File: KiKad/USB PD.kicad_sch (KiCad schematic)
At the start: 7 parts, among them J101 POWER_OUT, J4 USB_C_Receptacle_PowerOnly_6P, J5 USB_C_Receptacle_USB2.0_14P, Q301 Si2369, Q302 Si2338

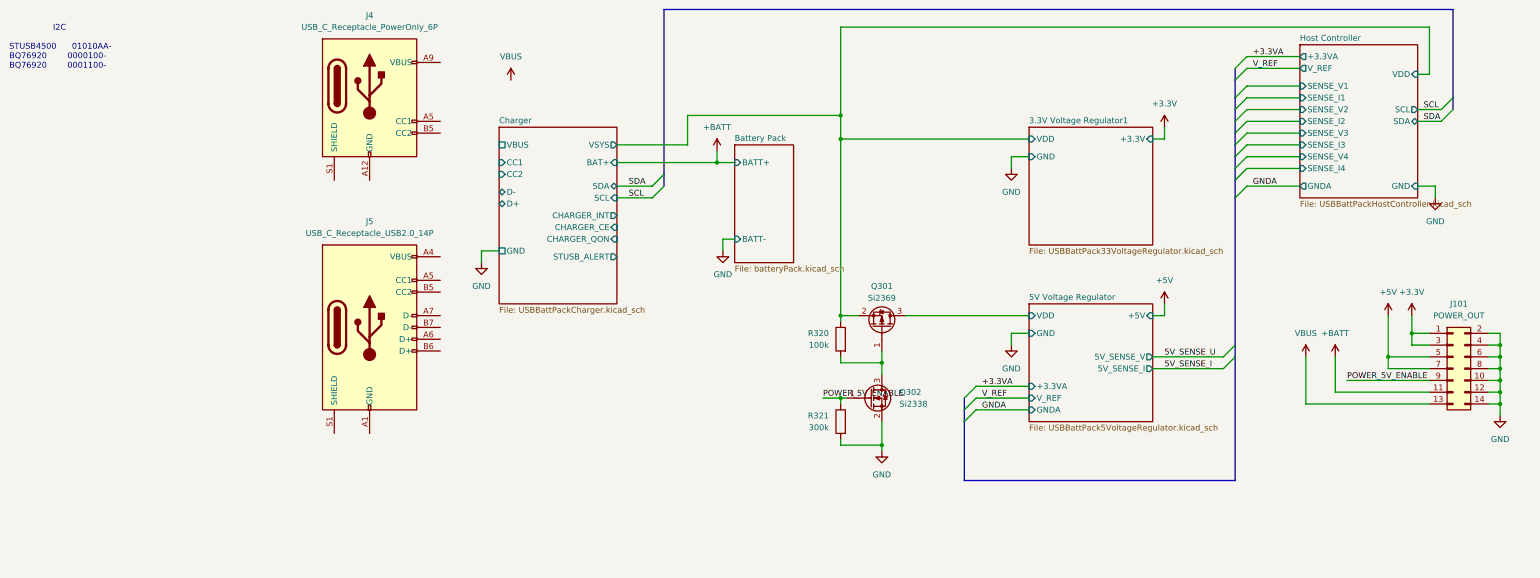
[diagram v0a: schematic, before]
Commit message: some work
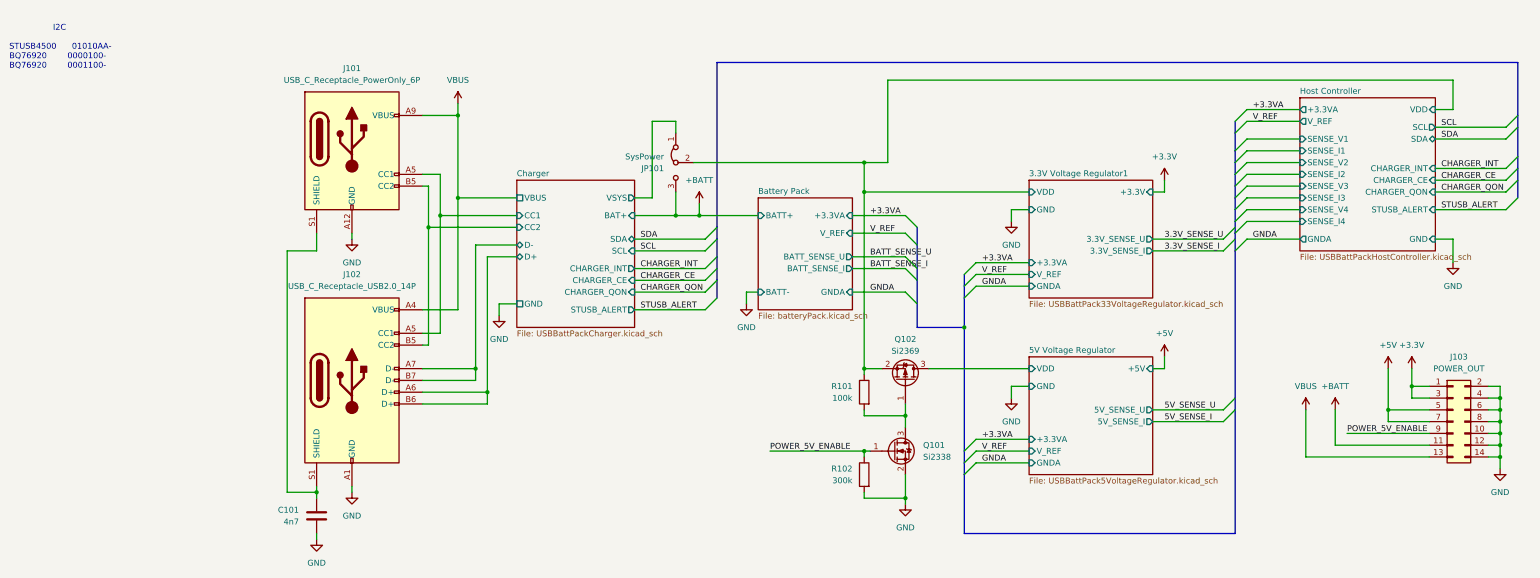
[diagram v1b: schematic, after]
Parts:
- added C101: 4n7, Capacitor_SMD:C_0805_2012Metric, symbol Device:C
- added JP101: SysPower, symbol Jumper:Jumper_3_Bridged12
- renumbered J4 to J101, J5 to J102, J101 to J103, Q302 to Q101, Q301 to Q102, R320 to R101, R321 to R102
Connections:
- net +BATT: now also JP101.3 (B)
- net 3.3V Voltage Regulator1/VDD: now also JP101.2 (C)
- net Charger/CC1: now also J101.A5 (CC1), J102.A5 (CC1)
- net Charger/CC2: now also J101.B5 (CC2), J102.B5 (CC2)
- net Charger/D+: now also J102.A6 (D+), J102.B6 (D+)
- net Charger/D-: now also J102.A7 (D-), J102.B7 (D-)
- net GND: now also J101.A12 (GND), J101.B12 (GND), J102.A1 (GND), J102.A12 (GND), J102.B1 (GND), J102.B12 (GND), C101.2
- net VBUS: now also J101.A9 (VBUS), J101.B9 (VBUS), J102.A4 (VBUS), J102.A9 (VBUS), J102.B4 (VBUS), J102.B9 (VBUS)
- net at J102.S1 (SHIELD): now also J101.S1 (SHIELD), C101.1
- new net Charger/VSYS: JP101.1 (A)
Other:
- sheet 3.3V Voltage Regulator1 ports: added +3.3VA, 3.3V_SENSE_I, 3.3V_SENSE_U, GNDA, V_REF; removed none
- sheet 5V Voltage Regulator ports: added 5V_SENSE_U; removed 5V_SENSE_V
- sheet Battery Pack ports: added +3.3VA, BATT_SENSE_I, BATT_SENSE_U, GNDA, V_REF; removed none
- sheet Host Controller ports: added CHARGER_CE, CHARGER_INT, CHARGER_QON, STUSB_ALERT; removed none
- moved on the sheet: J101, J102, J103, Q101, Q102, R101, R102
